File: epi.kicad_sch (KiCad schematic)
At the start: 29 parts, among them J1 Connector 1x12, J2 Connector 1x12, J3 Conn_01x05, J4 USB-C 2.0 mid-mount female co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, U1 ATmega32U4-M, Y1 Crystal_GND24_Small

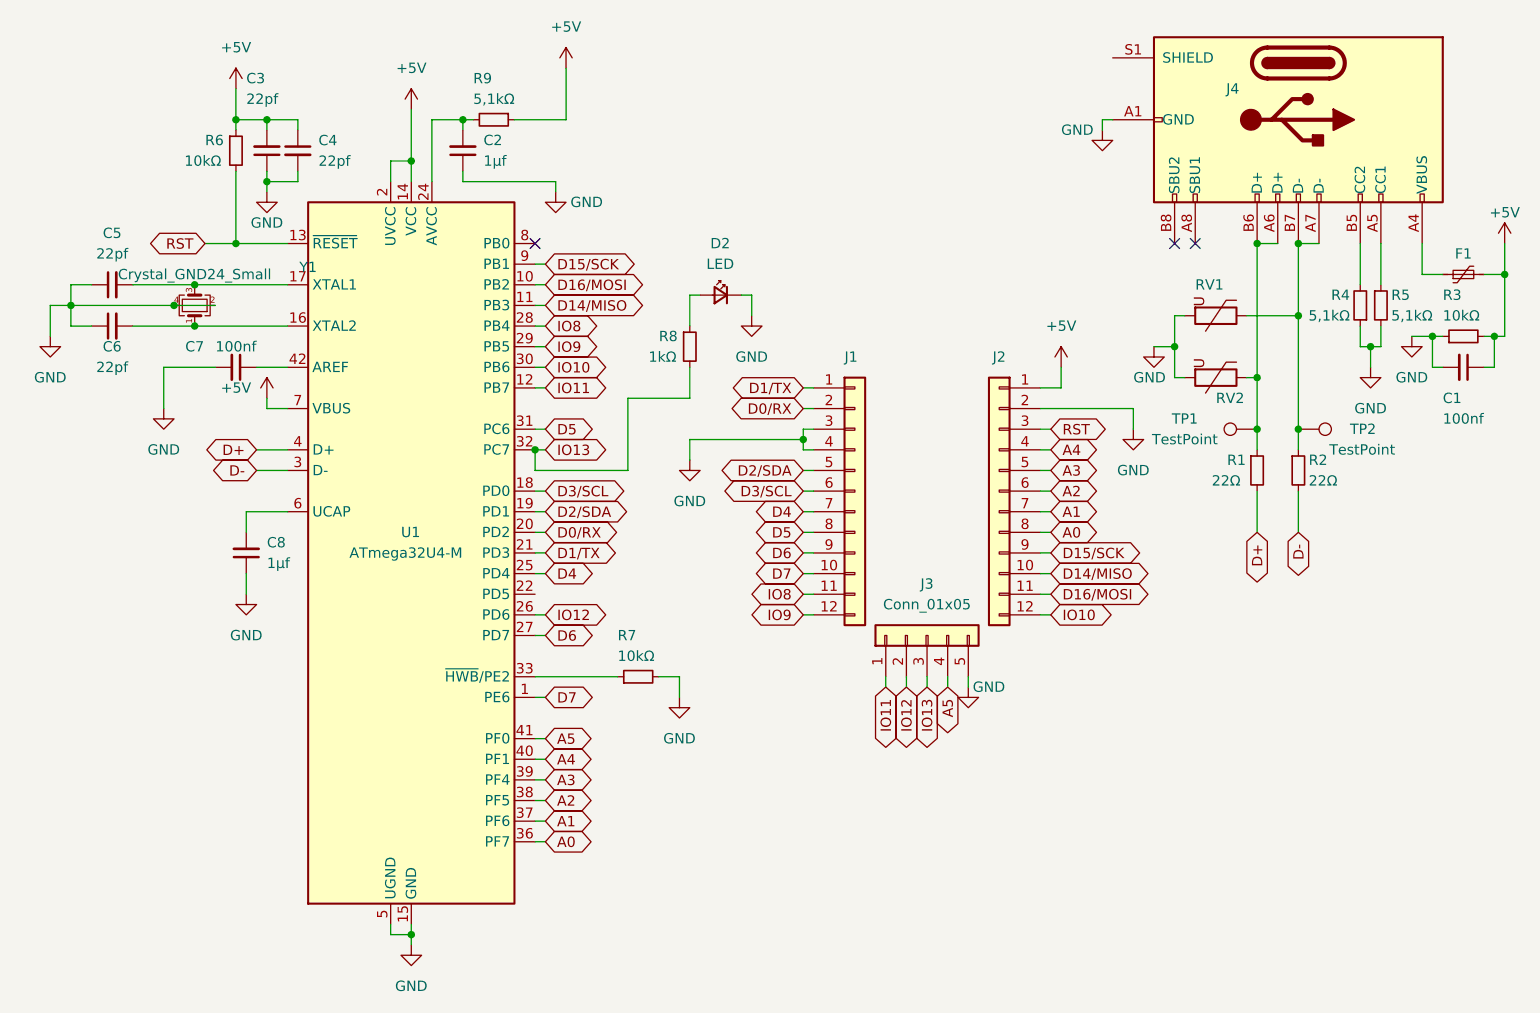
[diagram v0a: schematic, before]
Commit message: initial
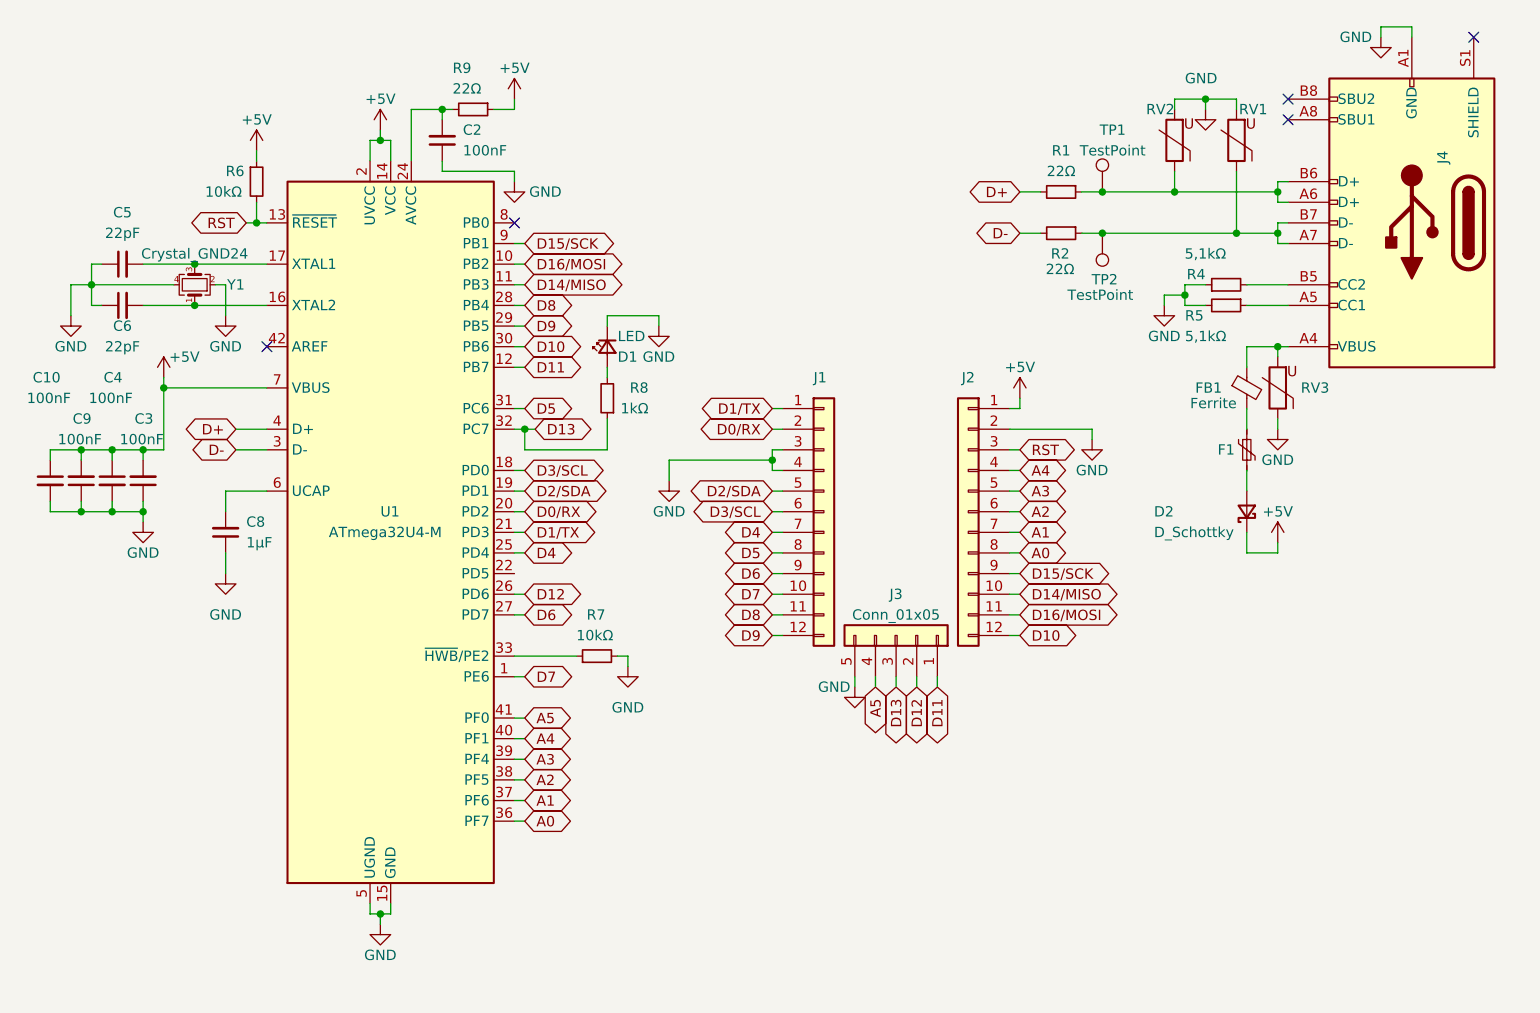
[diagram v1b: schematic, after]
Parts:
- removed C1, C7: 100nf, Capacitor_SMD:C_0402_1005Metric, symbol Device:C_Small
- removed R3: 10kΩ, Resistor_SMD:R_0402_1005Metric, symbol Device:R_Small
- added C10, C9: 100nF, Capacitor_SMD:C_0402_1005Metric, symbol Device:C_Small
- added D2: D_Schottky, DIY:SOD323_bättre, symbol Device:D_Schottky_Small
- added FB1: Ferrite, Resistor_SMD:R_0402_1005Metric, symbol Device:FerriteBead_Small
- added RV3: ESD protection varistor, Resistor_SMD:R_0402_1005Metric, symbol Device:Varistor
- C2: value 1µf -> 100nF
- C3, C4: value 22pf -> 100nF
- C5, C6: value 22pf -> 22pF
- C8: value 1µf -> 1µF
- R9: value 5,1kΩ -> 22Ω
- Y1: value Crystal_GND24_Small -> Crystal_GND24
- renumbered D2 to D1
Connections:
- net +5V: now also C10.1, C9.2, D2.1 (K); no longer F1.2
- net GND: now also C10.2, C9.1, RV3.1
- net at D1.2 (A): now also R8.2; no longer R8.1
- net at J4.A4 (VBUS), J4.A9 (VBUS), J4.B4 (VBUS)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: now also FB1.1, RV3.2; no longer F1.1
- net IO10 renamed D10
- net IO11 renamed D11
- net IO12 renamed D12
- net IO13 renamed D13
- net D13: now also R8.1; no longer R8.2
- net IO8 renamed D8
- net IO9 renamed D9
- new net: D2.2 (A), F1.2
- new net: F1.1, FB1.2
- no-connect marks 3 -> 5
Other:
- moved on the sheet: C2, C3, C4, C5, C6, C8, D1, F1, J1, J2, J3, J4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
